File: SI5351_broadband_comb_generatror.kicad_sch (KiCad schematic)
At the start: 10 parts, among them J1 Conn_Coaxial_Small, J2 Conn_Coaxial_Small, U1 Si5351C-B-GM, U2 ATmega328P-A, U3 FT232RL, U4 GALI-5, U5 KT2520K-T, U6 ISL3280ExHZ

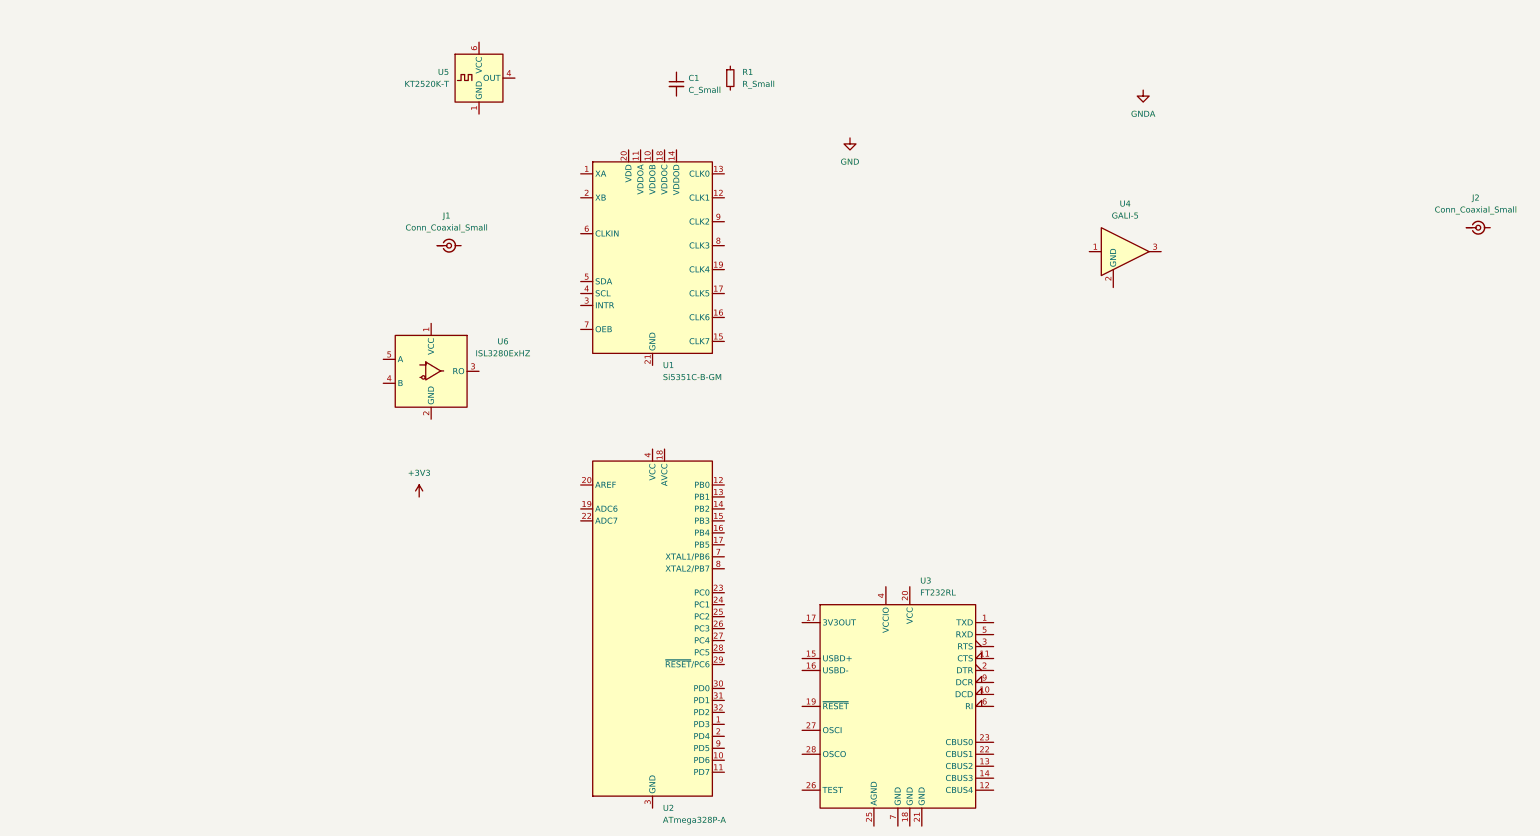
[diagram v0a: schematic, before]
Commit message: working on the schematic...
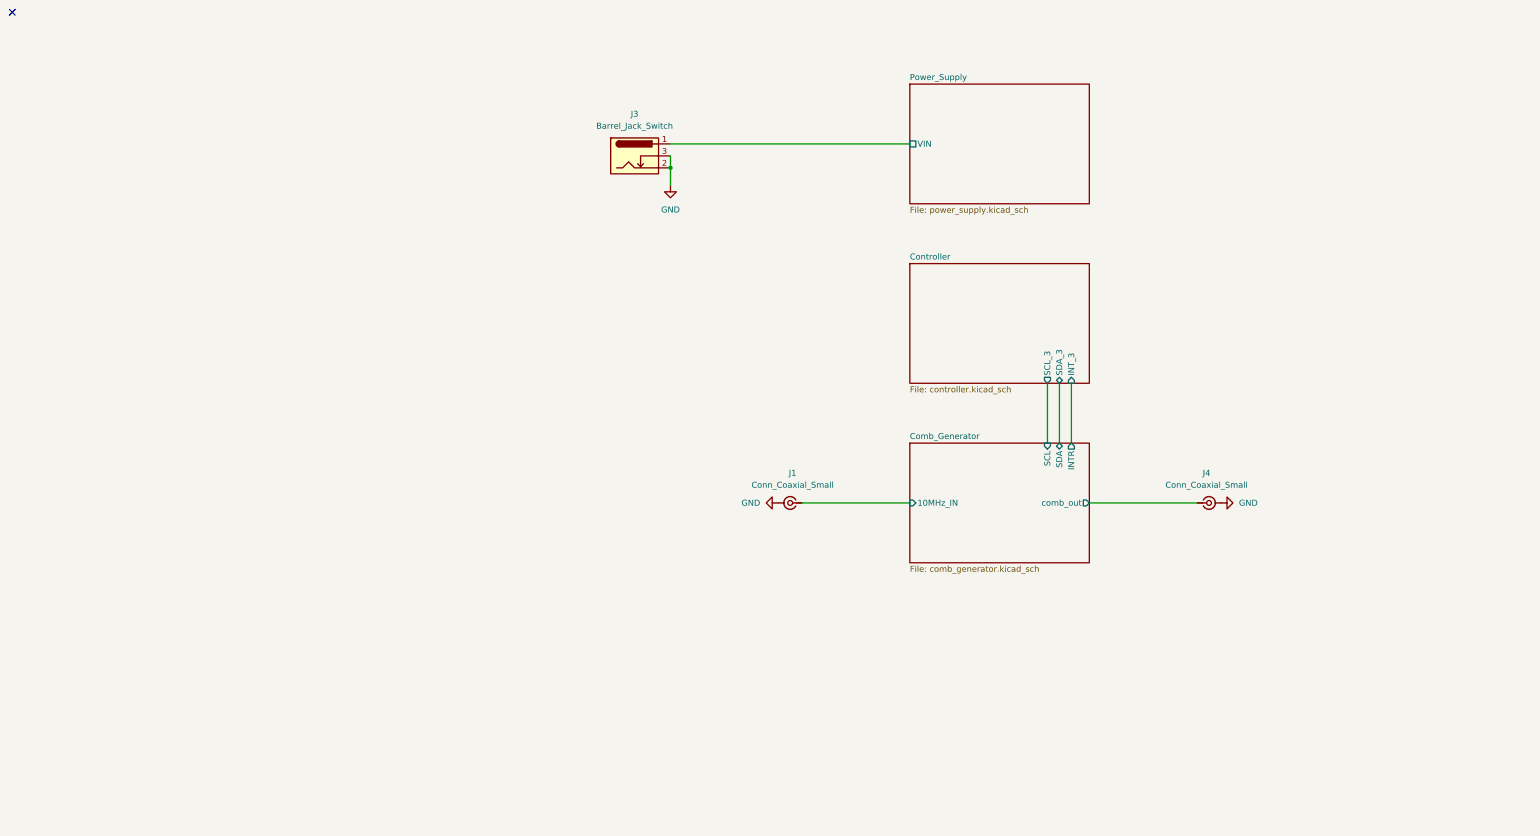
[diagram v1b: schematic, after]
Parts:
- removed C1: C_Small, Capacitor_SMD:C_0603_1608Metric_Pad1.08x0.95mm_HandSolder, symbol Device:C_Small
- removed J2: Conn_Coaxial_Small, Connector_Coaxial:SMA_Molex_73251-1153_EdgeMount_Horizontal, symbol Connector:Conn_Coaxial_Small
- removed R1: R_Small, Resistor_SMD:R_0603_1608Metric_Pad0.98x0.95mm_HandSolder, symbol Device:R_Small
- removed U1: Si5351C-B-GM, Package_DFN_QFN:QFN-20-1EP_4x4mm_P0.5mm_EP2.7x2.7mm, symbol Oscillator:Si5351C-B-GM
- removed U2: ATmega328P-A, Package_QFP:TQFP-32_7x7mm_P0.8mm, symbol MCU_Microchip_ATmega:ATmega328P-A
- removed U3: FT232RL, Package_SO:SSOP-28_5.3x10.2mm_P0.65mm, symbol Interface_USB:FT232RL
- removed U4: GALI-5, Package_TO_SOT_SMD:SOT-89-3, symbol RF_Amplifier:GALI-5
- removed U5: KT2520K-T, Oscillator:Oscillator_SMD_Kyocera_2520-6Pin_2.5x2.0mm, symbol Oscillator:KT2520K-T
- removed U6: ISL3280ExHZ, Package_TO_SOT_SMD:SOT-23-5_HandSoldering, symbol Interface_UART:ISL3280ExHZ
- added J3: Barrel_Jack_Switch, Connector_BarrelJack:BarrelJack_Wuerth_6941xx301002, symbol Connector:Barrel_Jack_Switch
- added J4: Conn_Coaxial_Small, Connector_Coaxial:SMA_Molex_73251-1153_EdgeMount_Horizontal, symbol Connector:Conn_Coaxial_Small
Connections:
- net GND: now also J1.2 (Ext), J3.2, J3.3, J4.2 (Ext)
- net Comb_Generator/10MHz_IN: now reaches J1.1 (In)
- new net Comb_Generator/comb_out: J4.1 (In)
- new net Power_Supply/VIN: J3.1
- no-connect marks 0 -> 1
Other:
- added sheet Comb_Generator (comb_generator.kicad_sch)
- added sheet Controller (controller.kicad_sch)
- added sheet Power_Supply (power_supply.kicad_sch)
